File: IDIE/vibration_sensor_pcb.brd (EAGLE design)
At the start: 61.3 x 43.4 mm, 63 parts, among them IC1 LORA-E5, IC2 STM32L071KBT6, IC3 FXLS8974CFR3, IC4 FXLS8971CFR1, IC5 DRV5032FBLPGM, IC6 FT234XD-T, J1 217182-0001, Q2 SI2305B-TP, Y1 ABS06-32.768KHZ-9-1-T

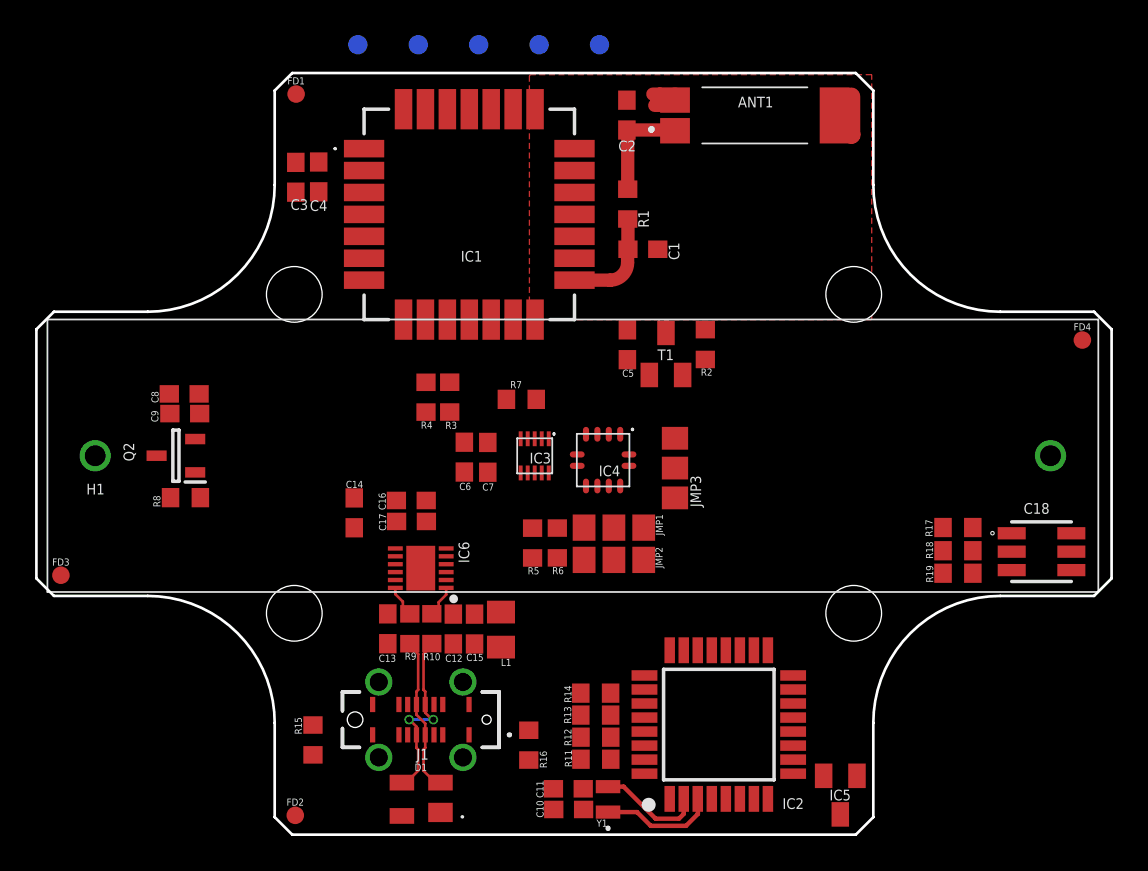
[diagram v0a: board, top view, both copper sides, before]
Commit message: ADD & UPDATE documentacion, modelado 3d y poco ruteo
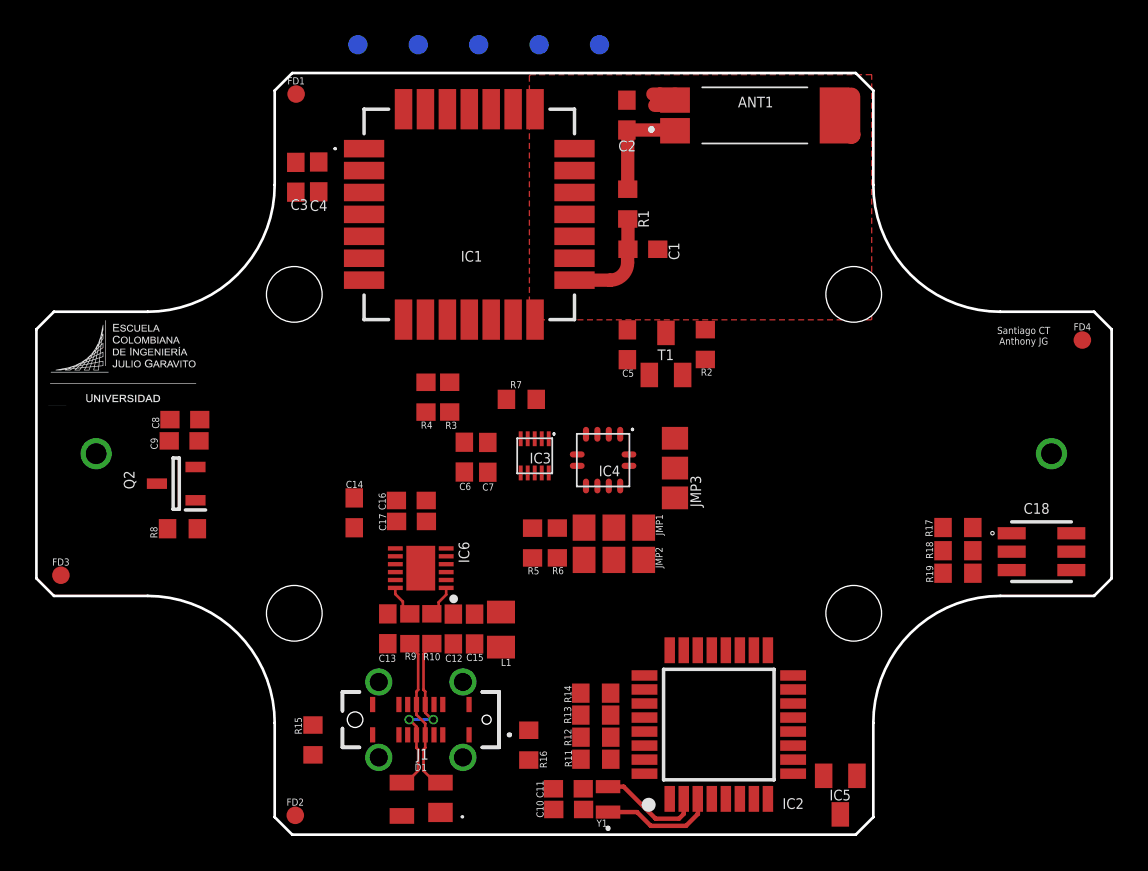
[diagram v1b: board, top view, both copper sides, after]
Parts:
- moved R8 1.78 mm to (8.40, 17.4)
- moved Q2 1.59 mm to (8.05, 20.0)
- moved C9 1.56 mm to (8.50, 22.5)
- moved C8 1.47 mm to (8.54, 23.7)
- moved H1 0.13 mm to (3.48, 21.7), flipped to the bottom, turned to 180 degrees
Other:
- board text added: "C:/Users/Scort/Downloads/Logotipo-Escuela-Colombiana-de-Ingeniería-Julio-Garavito-1.bmp"
- board text added: "Santiago CT Anthony JG"
